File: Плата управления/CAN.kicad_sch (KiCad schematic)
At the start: 20 parts

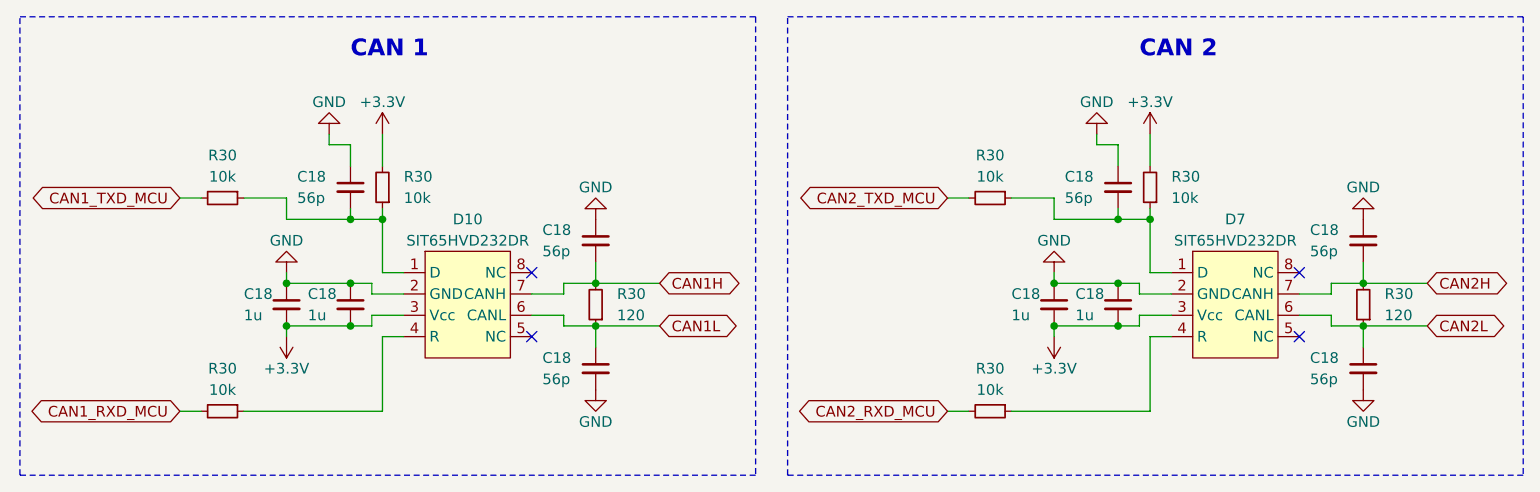
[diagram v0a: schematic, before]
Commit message: Новый контур платы
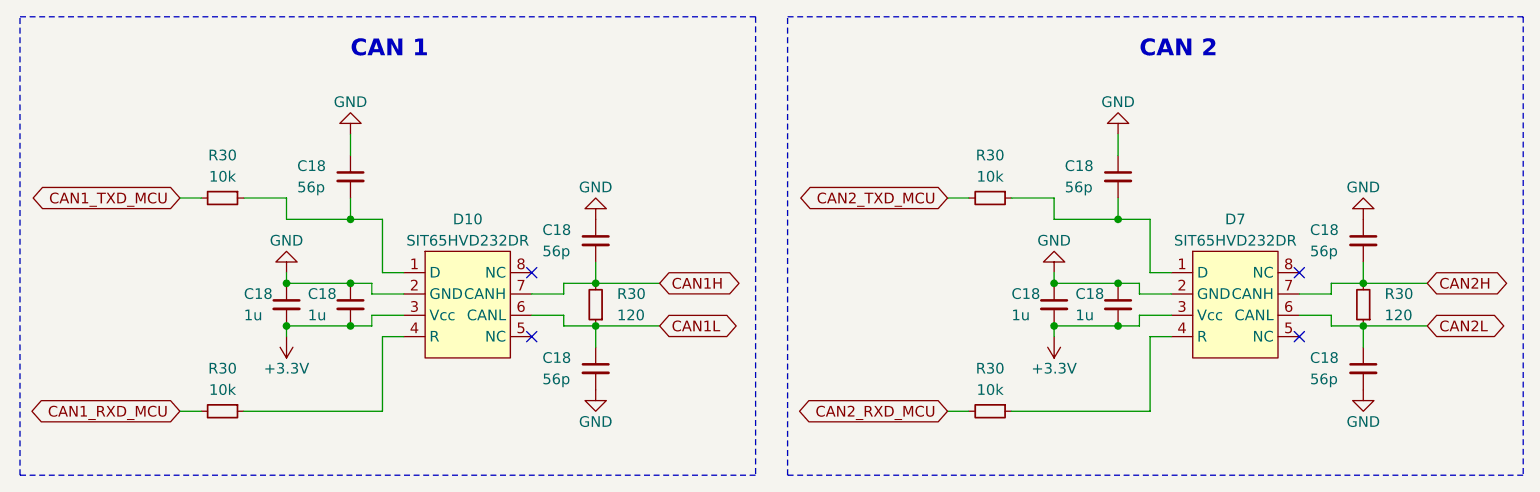
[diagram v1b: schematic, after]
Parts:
- removed R30 (x2): 10k, Resistor_SMD:R_0603_1608Metric_Pad0.98x0.95mm_HandSolder, symbol Device:R_Small
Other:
- moved on the sheet: C18
